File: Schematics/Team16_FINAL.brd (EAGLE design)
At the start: 33 x 35.2 mm, 20 parts, among them J1 AVR_SPI_PROG_3X2PTH, U1 ATMEGA328P_TQFP, U3 ADXL345, U4 3.3V/150mA, Y1 8MHz

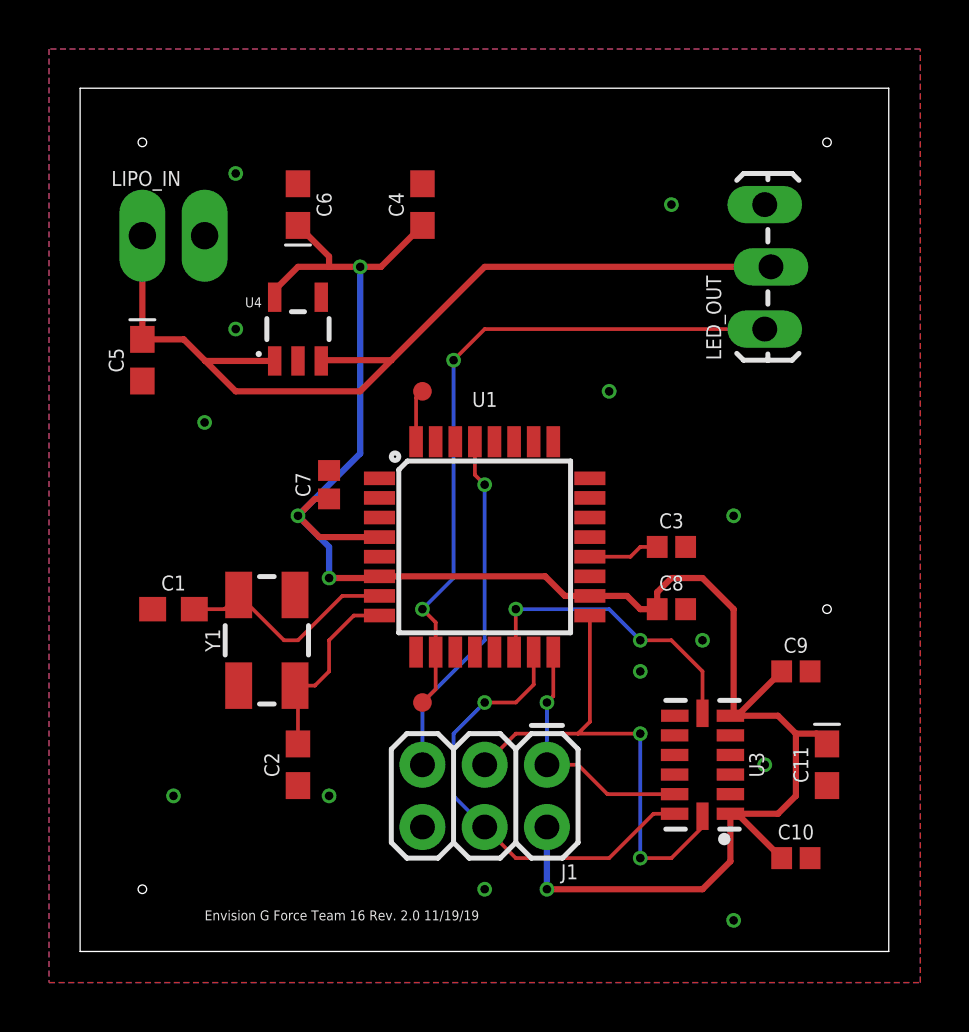
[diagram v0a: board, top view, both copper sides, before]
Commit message: Add files via upload
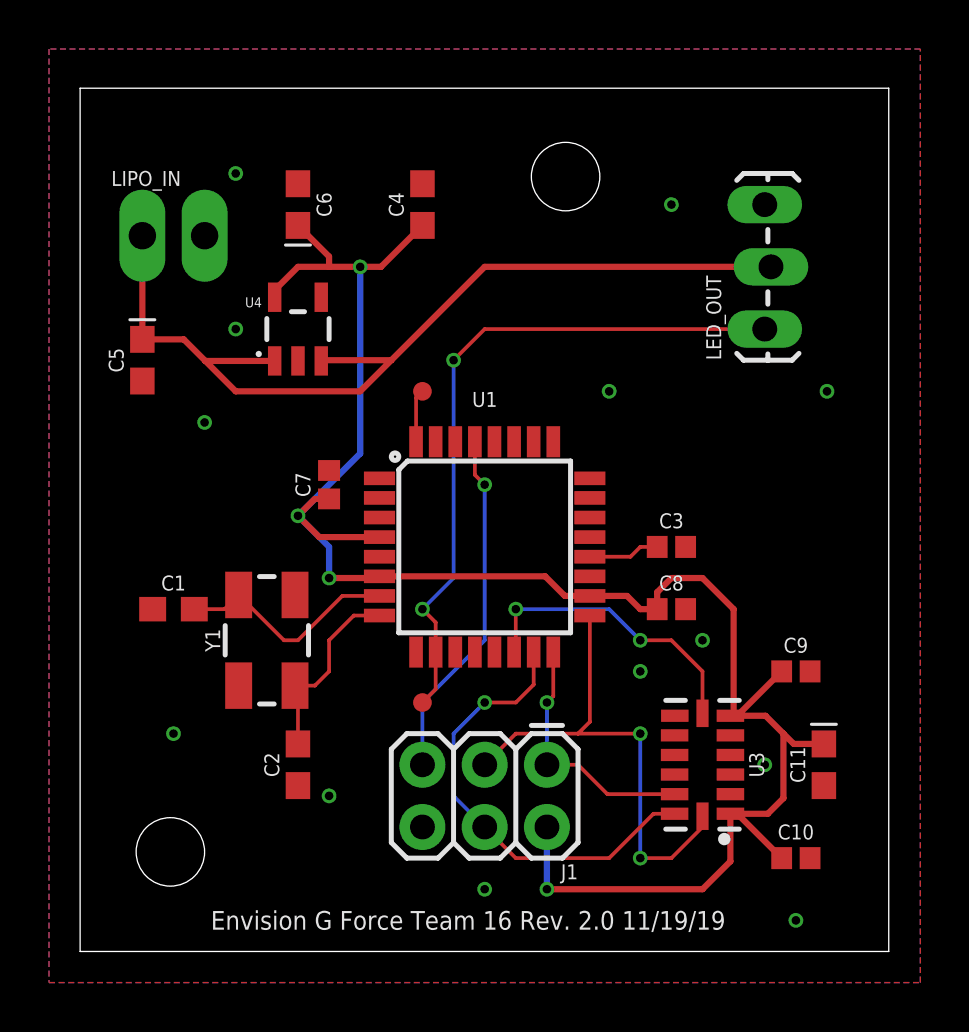
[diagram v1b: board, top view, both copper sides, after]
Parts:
- moved C11 0.13 mm to (30.4, 6.35)
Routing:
- net VCC: track 79.5 -> 79.0 mm
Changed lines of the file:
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@@
 <setting verticaltext="up"/>
 </settings>
-<grid distance="50" unitdist="mil" unit="mil" style="lines" multiple="1" display="no" altdistance="5" altunitdist="mil" altunit="mil"/>
+<grid distance="5" unitdist="mil" unit="mil" style="lines" multiple="1" display="no" altdistance="5" altunitdist="mil" altunit="mil"/>
 <layers>
 <layer number="1" name="Top" color="4" fill="1" visible="yes" active="yes"/>
@@
 <wire x1="33" y1="33.96" x2="0" y2="33.96" width="0" layer="20"/>
 <wire x1="0" y1="33.96" x2="0" y2="-1.27" width="0" layer="20"/>
-<hole x="2.54" y="1.27" drill="0.35"/>
-<hole x="2.54" y="31.75" drill="0.35"/>
-<hole x="30.48" y="31.75" drill="0.35"/>
-<text x="5.08" y="0" size="0.4064" layer="21">Envision G Force Team 16 Rev. 2.0 11/19/19</text>
-<hole x="30.48" y="12.7" drill="0.35"/>
+<hole x="3.683" y="2.794" drill="2.794"/>
+<hole x="19.812" y="30.353" drill="2.794"/>
+<text x="5.334" y="-0.381" size="0.762" layer="21">Envision G Force Team 16 Rev. 2.0 11/19/19</text>
 </plain>
 <attributes>
@@
 <attribute name="PROD_ID" value="CAP-12416" x="29.21" y="2.54" size="0.4064" layer="27" display="off"/>
 </element>
-<element name="C11" library="SparkFun-Capacitors" package="0603-POLAR" value="10uF" x="30.48" y="6.35" smashed="yes" rot="R90">
-<attribute name="NAME" x="29.718" y="6.35" size="0.6096" layer="25" font="vector" ratio="20" rot="R90" align="bottom-center"/>
-<attribute name="PROD_ID" value="CAP-13210" x="30.48" y="6.35" size="0.4064" layer="27" rot="R90" display="off"/>
+<element name="C11" library="SparkFun-Capacitors" package="0603-POLAR" value="10uF" x="30.353" y="6.35" smashed="yes" rot="R90">
+<attribute name="NAME" x="29.591" y="6.35" size="0.6096" layer="25" font="vector" ratio="20" rot="R90" align="bottom-center"/>
+<attribute name="PROD_ID" value="CAP-13210" x="30.353" y="6.35" size="0.4064" layer="27" rot="R90" display="off"/>
 </element>
 </elements>
@@
 <contactref element="C6" pad="-"/>
 <via x="6.35" y="24.13" extent="1-16" drill="0.35"/>
-<via x="26.67" y="16.51" extent="1-16" drill="0.35"/>
+<via x="30.48" y="21.59" extent="1-16" drill="0.35"/>
 <via x="5.08" y="20.32" extent="1-16" drill="0.35"/>
 <contactref element="C8" pad="2"/>
@@
 <via x="22.86" y="10.16" extent="1-16" drill="0.35"/>
 <via x="21.59" y="21.59" extent="1-16" drill="0.35"/>
-<via x="3.81" y="5.08" extent="1-16" drill="0.35"/>
+<via x="3.81" y="7.62" extent="1-16" drill="0.35"/>
 <via x="16.51" y="1.27" extent="1-16" drill="0.35"/>
 <contactref element="C11" pad="-"/>
 <contactref element="C10" pad="2"/>
 <contactref element="C9" pad="2"/>
-<via x="26.67" y="0" extent="1-16" drill="0.35"/>
+<via x="29.21" y="0" extent="1-16" drill="0.35"/>
 </signal>
 <signal name="N$1">
@@
 <wire x1="25.4" y1="1.27" x2="26.5381" y2="2.4081" width="0.254" layer="1"/>
 <wire x1="26.5381" y1="2.4081" x2="26.5381" y2="4.35" width="0.254" layer="1"/>
-<wire x1="29.21" y1="7.62" x2="28.48" y2="8.35" width="0.254" layer="1"/>
-<wire x1="29.21" y1="7.62" x2="29.21" y2="5.08" width="0.254" layer="1"/>
-<wire x1="29.21" y1="5.08" x2="28.48" y2="4.35" width="0.254" layer="1"/>
-<wire x1="28.48" y1="4.35" x2="26.82" y2="4.35" width="0.254" layer="1"/>
+<wire x1="27.972" y1="8.35" x2="28.702" y2="7.62" width="0.254" layer="1"/>
 <via x="11.43" y="26.67" extent="1-16" drill="0.35"/>
 <via x="8.89" y="16.51" extent="1-16" drill="0.35"/>
 <via x="10.16" y="13.97" extent="1-16" drill="0.35"/>
-<wire x1="26.67" y1="4.35" x2="26.5381" y2="4.35" width="0.254" layer="1"/>
+<wire x1="28.067" y1="4.35" x2="26.82" y2="4.35" width="0.254" layer="1"/>
 <wire x1="11.43" y1="26.67" x2="11.43" y2="19.05" width="0.254" layer="16"/>
 <wire x1="11.43" y1="19.05" x2="8.89" y2="16.51" width="0.254" layer="16"/>
@@
 <wire x1="7.94" y1="25.4301" x2="7.94" y2="25.72" width="0.254" layer="1"/>
 <wire x1="7.94" y1="25.72" x2="8.89" y2="26.67" width="0.254" layer="1"/>
-<wire x1="28.48" y1="8.35" x2="26.82" y2="8.35" width="0.254" layer="1"/>
+<wire x1="27.972" y1="8.35" x2="26.82" y2="8.35" width="0.254" layer="1"/>
 <wire x1="26.67" y1="8.35" x2="26.5381" y2="8.35" width="0.254" layer="1"/>
 <wire x1="26.67" y1="12.7" x2="26.67" y2="8.35" width="0.254" layer="1"/>
@@
 <contactref element="C10" pad="1"/>
 <contactref element="C9" pad="1"/>
-<wire x1="30.48" y1="7.2" x2="30.06" y2="7.62" width="0.254" layer="1"/>
-<wire x1="30.06" y1="7.62" x2="29.21" y2="7.62" width="0.254" layer="1"/>
 <wire x1="28.63" y1="10.16" x2="26.82" y2="8.35" width="0.254" layer="1"/>
 <wire x1="26.82" y1="8.35" x2="26.67" y2="8.35" width="0.254" layer="1"/>
 <wire x1="28.63" y1="2.54" x2="26.82" y2="4.35" width="0.254" layer="1"/>
-<wire x1="26.82" y1="4.35" x2="26.67" y2="4.35" width="0.254" layer="1"/>
+<wire x1="26.82" y1="4.35" x2="26.5381" y2="4.35" width="0.254" layer="1"/>
+<wire x1="28.702" y1="7.62" x2="28.702" y2="4.985" width="0.254" layer="1"/>
+<wire x1="28.702" y1="4.985" x2="28.067" y2="4.35" width="0.254" layer="1"/>
+<wire x1="30.353" y1="7.2" x2="29.122" y2="7.2" width="0.254" layer="1"/>
+<wire x1="29.122" y1="7.2" x2="28.702" y2="7.62" width="0.254" layer="1"/>
 </signal>
 </signals>
